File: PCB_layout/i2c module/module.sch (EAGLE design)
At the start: 5 parts, among them IC1 ATTINY85-20SU, J1 M20-9980346

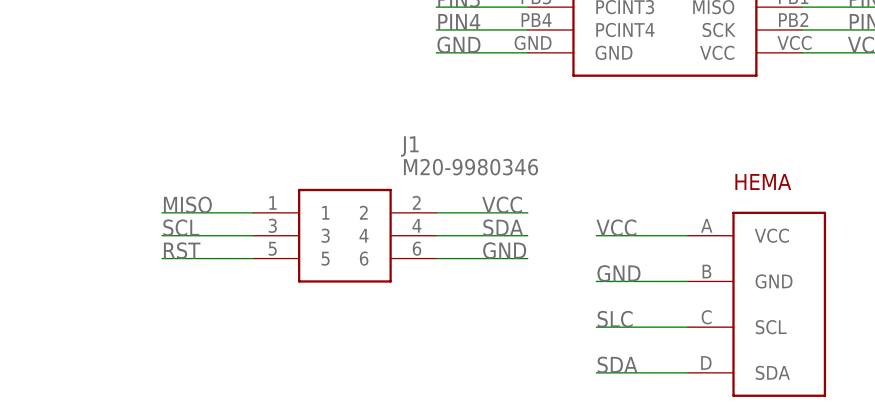
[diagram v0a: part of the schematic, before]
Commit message: i2c, lbr updates
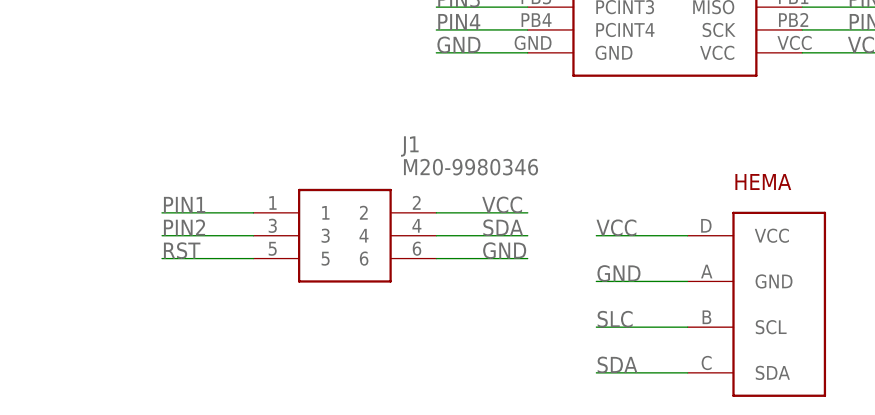
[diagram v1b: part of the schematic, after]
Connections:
- removed net MISO: J1.1
- removed net SCL: J1.3
- net PIN1: now also J1.1
- net PIN2: now also J1.3
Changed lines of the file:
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@@
-</segment>
-</net>
-<net name="MISO" class="0">
-<segment>
-<pinref part="J1" gate="G$1" pin="1"/>
-<wire x1="5.08" y1="58.42" x2="-5.08" y2="58.42" width="0.1524" layer="91"/>
-<label x="-5.08" y="58.42" size="1.778" layer="95"/>
-</segment>
-</net>
-<net name="SCL" class="0">
-<segment>
-<pinref part="J1" gate="G$1" pin="3"/>
-<wire x1="5.08" y1="55.88" x2="-5.08" y2="55.88" width="0.1524" layer="91"/>
-<label x="-5.08" y="55.88" size="1.778" layer="95"/>
 </segment>
 </net>
@@
 <label x="71.12" y="81.28" size="1.778" layer="95"/>
 </segment>
+<segment>
+<pinref part="J1" gate="G$1" pin="1"/>
+<wire x1="5.08" y1="58.42" x2="-5.08" y2="58.42" width="0.1524" layer="91"/>
+<label x="-5.08" y="58.42" size="1.778" layer="95"/>
+</segment>
 </net>
 <net name="PIN2" class="0">
@@
 <wire x1="66.04" y1="78.74" x2="76.2" y2="78.74" width="0.1524" layer="91"/>
 <label x="71.12" y="78.74" size="1.778" layer="95"/>
+</segment>
+<segment>
+<pinref part="J1" gate="G$1" pin="3"/>
+<wire x1="5.08" y1="55.88" x2="-5.08" y2="55.88" width="0.1524" layer="91"/>
+<label x="-5.08" y="55.88" size="1.778" layer="95"/>
 </segment>
 </net>
@@
 </drawing>
 <compatibility>
+<note version="6.3" minversion="6.2.2" severity="warning">
+Since Version 6.2.2 text objects can contain more than one line,
+which will not be processed correctly with this version.
+</note>
 <note version="8.2" severity="warning">
 Since Version 8.2, EAGLE supports online libraries. The ids

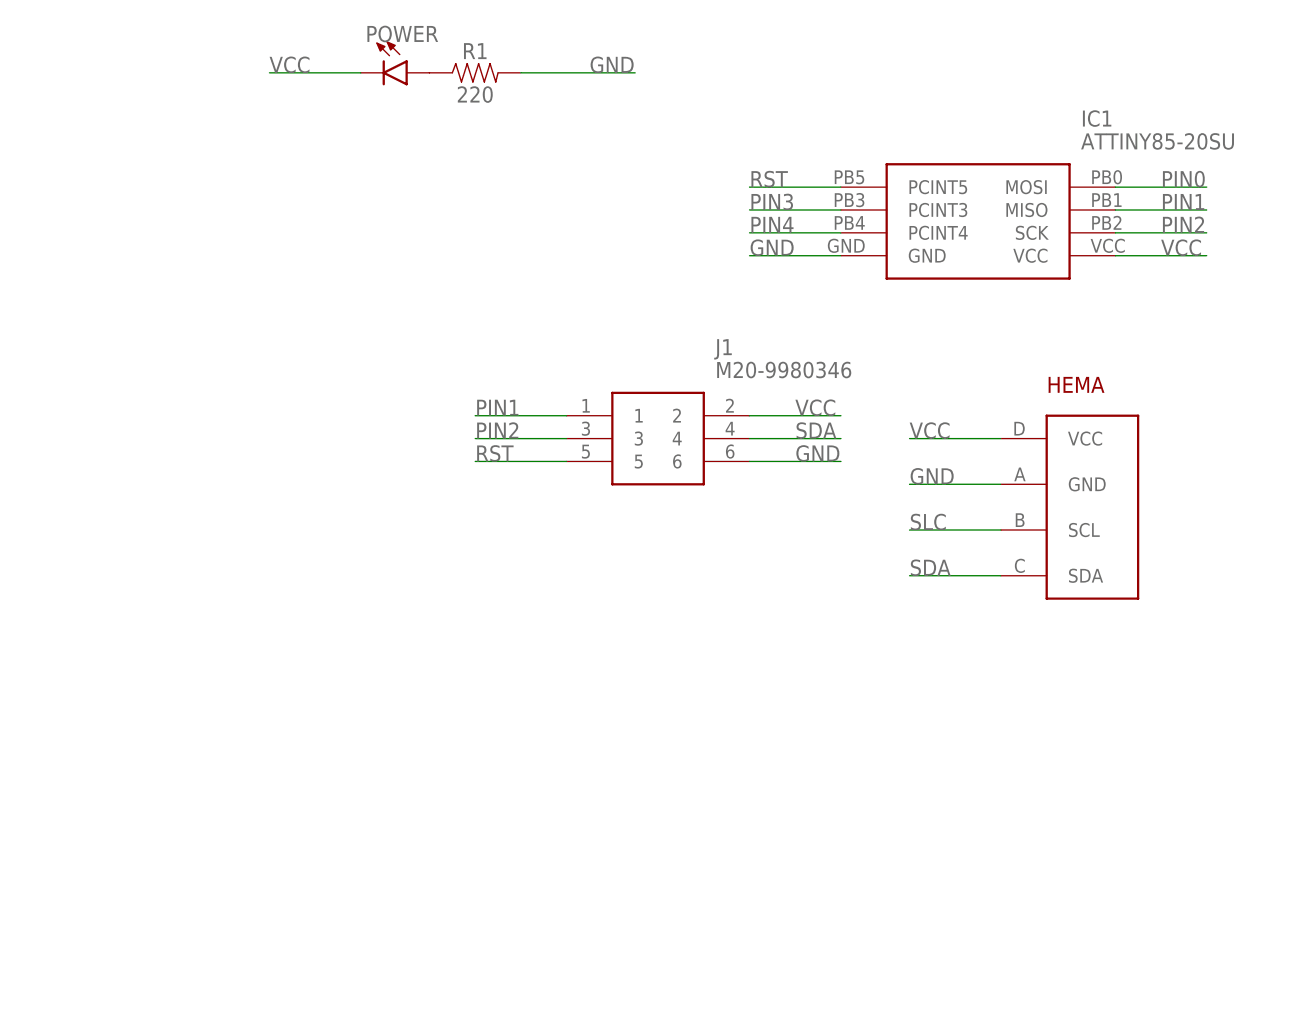
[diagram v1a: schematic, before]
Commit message: PCB design/lib updates
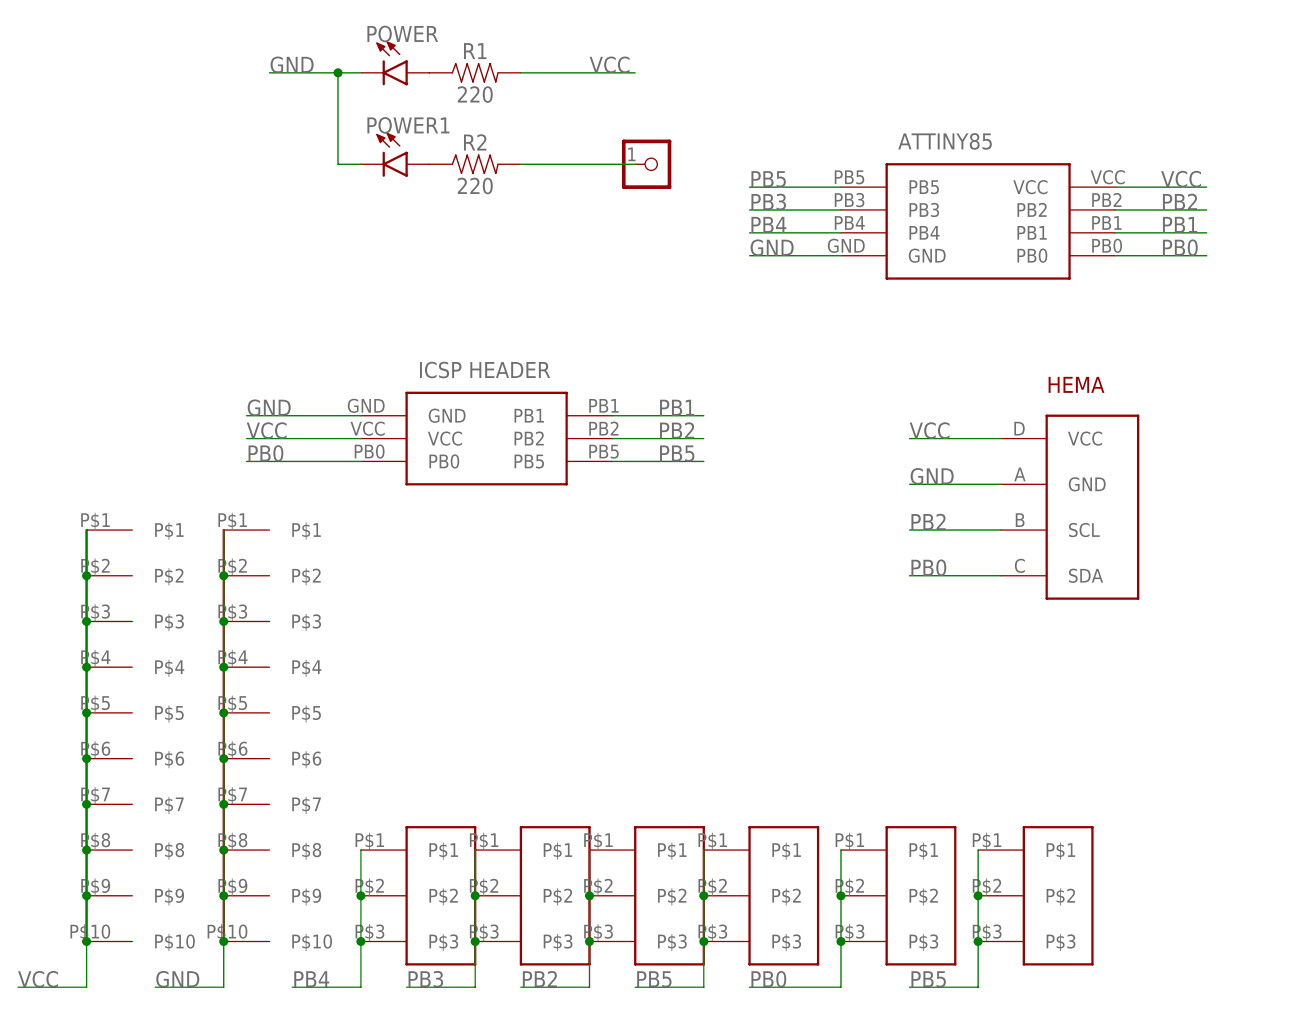
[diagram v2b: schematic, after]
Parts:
- added 0, 1, 2, 3, 4, 5: 3X-PADS-CONNECTED, BadgeParts:3X-PADS-CONNECTED
- added GND, VCC: 10X-PADS, BadgeParts:10X-PADS
- added P1: PROTO_VIAS_01X01-1.2, dp_devices:PROTO_VIAS_01X01-1.2
- added POWER1: (no value), SparkFun-LED:LED3MM
- added R2: 220, SparkFun-Resistors:RESISTORAXIAL-0.3
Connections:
- removed net PIN0: IC1.MOSI
- removed net PIN1: IC1.MISO, J1.1
- removed net PIN2: IC1.SCK, J1.3
- removed net PIN3: IC1.PCINT3
- removed net PIN4: IC1.PCINT4
- removed net RST: IC1.PCINT5, J1.5
- removed net SDA: J1.4, U$1.SDA
- removed net SLC: U$1.SCL
- new net N$1: POWER1.A, R2.1
- new net N$2: P1.1, R2.2
- new net PB0: 0.P$1, 0.P$2, 0.P$3, IC1.PB0, J1.PB0, U$1.SDA
- new net PB1: IC1.PB1, J1.PB1
- new net PB2: 2.P$1, 2.P$2, 2.P$3, IC1.PB2, J1.PB2, U$1.SCL
- new net PB3: 3.P$1, 3.P$2, 3.P$3, IC1.PB3
- new net PB4: 4.P$1, 4.P$2, 4.P$3, IC1.PB4
- new net PB5: 1.P$1, 1.P$2, 1.P$3, 5.P$1, 5.P$2, 5.P$3, IC1.PB5, J1.PB5
- net GND: now also GND.P$1, GND.P$10, GND.P$2, GND.P$3, GND.P$4, GND.P$5, GND.P$6, GND.P$7, GND.P$8, GND.P$9, J1.GND, POWER.C, POWER1.C; no longer J1.6, R1.2
- net VCC: now also J1.VCC, R1.2, VCC.P$1, VCC.P$10, VCC.P$2, VCC.P$3, VCC.P$4, VCC.P$5, VCC.P$6, VCC.P$7, VCC.P$8, VCC.P$9; no longer J1.2, POWER.C

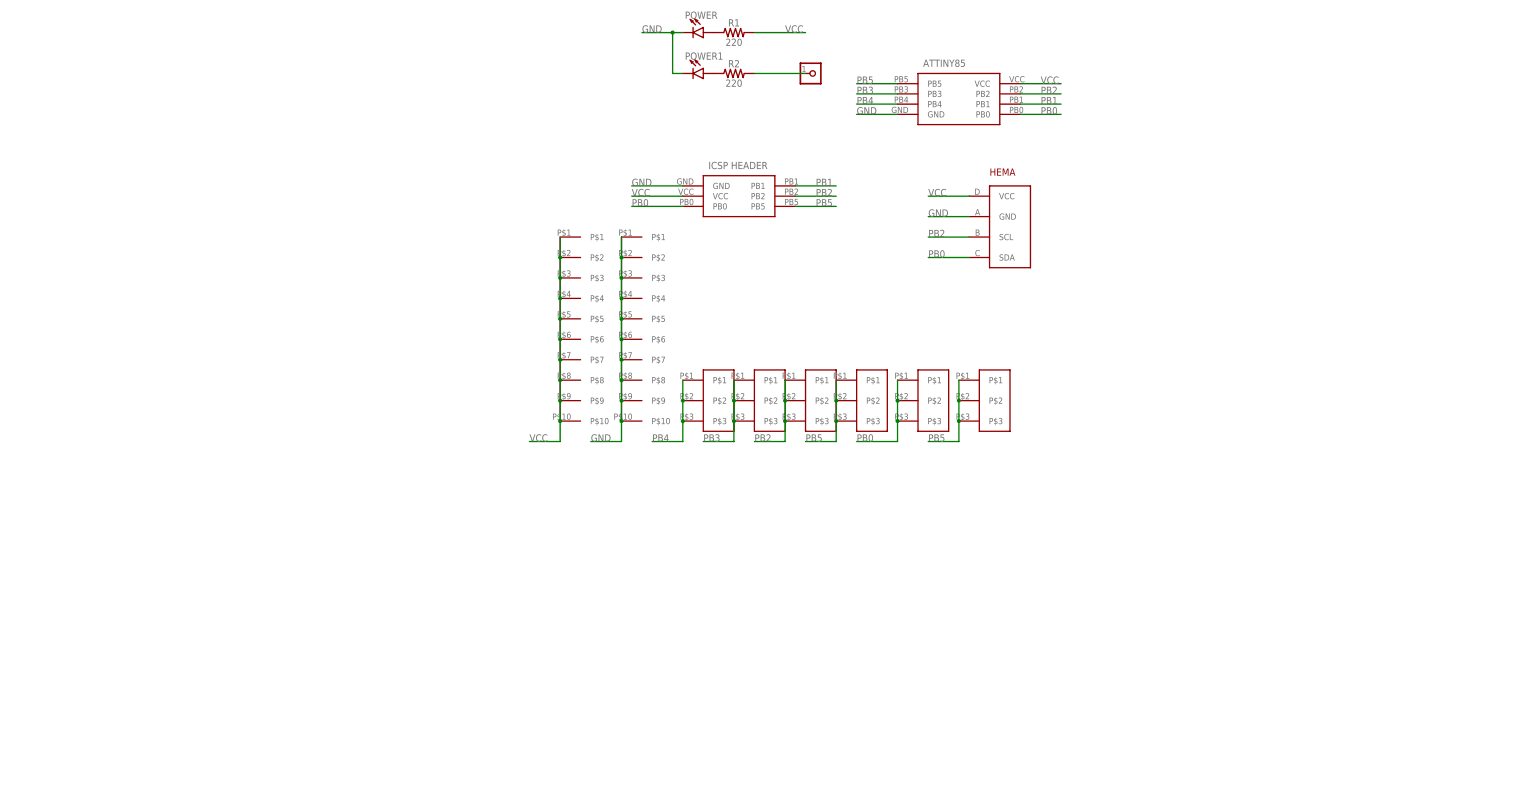
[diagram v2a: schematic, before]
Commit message: first i2c dongle iteration panelized
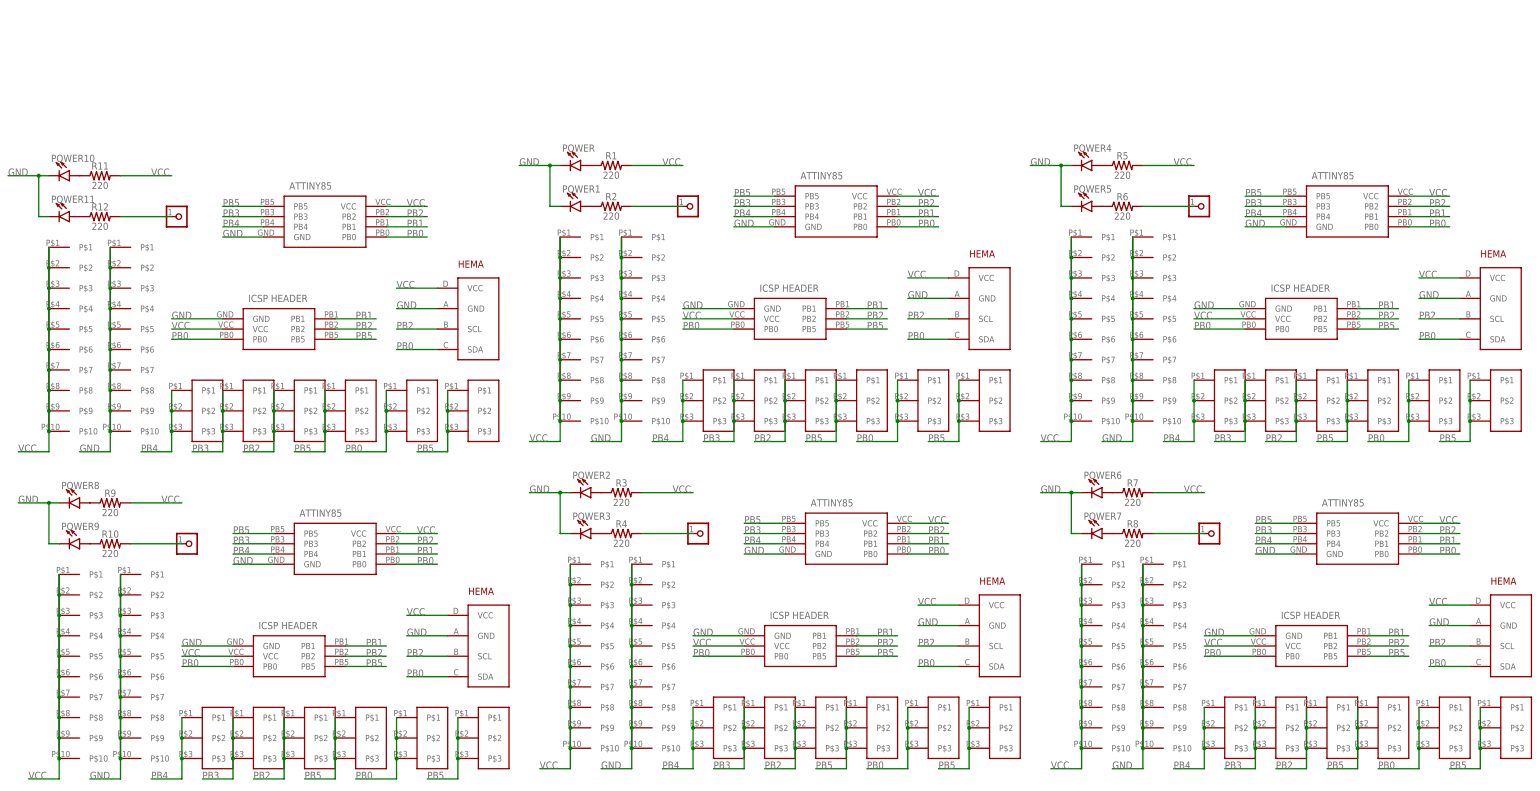
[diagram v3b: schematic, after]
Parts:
- added 10, 11, 12, 13, 14, 15, 16, 17, 18, 19, 20, 21, 22, 23, 24, 25, 26, 27, 28, 29, 30, 31, 32, 33, 34, 35, 6, 7, 8, 9: 3X-PADS-CONNECTED, BadgeParts:3X-PADS-CONNECTED
- added GND1, GND2, GND3, GND4, GND5, VCC1, VCC2, VCC3, VCC4, VCC5: 10X-PADS, BadgeParts:10X-PADS
- added IC2, IC3, IC4, IC5, IC6: ATTINY85-20SU, BadgeParts:ATTINY85-20SU
- added J2, J3, J4, J5, J6: M20-9980346, BadgeParts:M20-9980346
- added P2, P3, P4, P5, P6: PROTO_VIAS_01X01-1.2, dp_devices:PROTO_VIAS_01X01-1.2
- added POWER10, POWER11, POWER2, POWER3, POWER4, POWER5, POWER6, POWER7, POWER8, POWER9: (no value), SparkFun-LED:LED3MM
- added R10, R11, R12, R3, R4, R5, R6, R7, R8, R9: 220, SparkFun-Resistors:RESISTORAXIAL-0.3
- added U$2, U$3, U$4, U$5, U$6: HEMA-I2C, BadgeParts:HEMA-I2C
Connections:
- new net N$10: POWER7.A, R8.1
- new net N$12: P4.1, R8.2
- new net N$13: POWER8.A, R9.1
- new net N$14: POWER9.A, R10.1
- new net N$15: P5.1, R10.2
- new net N$16: POWER10.A, R11.1
- new net N$17: POWER11.A, R12.1
- new net N$18: P6.1, R12.2
- new net N$3: POWER2.A, R3.1
- new net N$4: POWER3.A, R4.1
- new net N$5: P2.1, R4.2
- new net N$6: POWER4.A, R5.1
- new net N$7: POWER5.A, R6.1
- new net N$8: P3.1, R6.2
- new net N$9: POWER6.A, R7.1
- net GND: now also GND1.P$1, GND1.P$10, GND1.P$2, GND1.P$3, GND1.P$4, GND1.P$5, GND1.P$6, GND1.P$7, GND1.P$8, GND1.P$9, GND2.P$1, GND2.P$10, GND2.P$2, GND2.P$3, GND2.P$4, GND2.P$5, GND2.P$6, GND2.P$7, GND2.P$8, GND2.P$9, GND3.P$1, GND3.P$10, GND3.P$2, GND3.P$3, GND3.P$4, GND3.P$5, GND3.P$6, GND3.P$7, GND3.P$8, GND3.P$9, GND4.P$1, GND4.P$10, GND4.P$2, GND4.P$3, GND4.P$4, GND4.P$5, GND4.P$6, GND4.P$7, GND4.P$8, GND4.P$9, GND5.P$1, GND5.P$10, GND5.P$2, GND5.P$3, GND5.P$4, GND5.P$5, GND5.P$6, GND5.P$7, GND5.P$8, GND5.P$9, IC2.GND, IC3.GND, IC4.GND, IC5.GND, IC6.GND, J2.GND, J3.GND, J4.GND, J5.GND, J6.GND, POWER10.C, POWER11.C, POWER2.C, POWER3.C, POWER4.C, POWER5.C, POWER6.C, POWER7.C, POWER8.C, POWER9.C, U$2.GND, U$3.GND, U$4.GND, U$5.GND, U$6.GND
- net PB0: now also 10.P$1, 10.P$2, 10.P$3, 16.P$1, 16.P$2, 16.P$3, 22.P$1, 22.P$2, 22.P$3, 28.P$1, 28.P$2, 28.P$3, 34.P$1, 34.P$2, 34.P$3, IC2.PB0, IC3.PB0, IC4.PB0, IC5.PB0, IC6.PB0, J2.PB0, J3.PB0, J4.PB0, J5.PB0, J6.PB0, U$2.SDA, U$3.SDA, U$4.SDA, U$5.SDA, U$6.SDA
- net PB1: now also IC2.PB1, IC3.PB1, IC4.PB1, IC5.PB1, IC6.PB1, J2.PB1, J3.PB1, J4.PB1, J5.PB1, J6.PB1
- net PB2: now also 14.P$1, 14.P$2, 14.P$3, 20.P$1, 20.P$2, 20.P$3, 26.P$1, 26.P$2, 26.P$3, 32.P$1, 32.P$2, 32.P$3, 8.P$1, 8.P$2, 8.P$3, IC2.PB2, IC3.PB2, IC4.PB2, IC5.PB2, IC6.PB2, J2.PB2, J3.PB2, J4.PB2, J5.PB2, J6.PB2, U$2.SCL, U$3.SCL, U$4.SCL, U$5.SCL, U$6.SCL
- net PB3: now also 13.P$1, 13.P$2, 13.P$3, 19.P$1, 19.P$2, 19.P$3, 25.P$1, 25.P$2, 25.P$3, 31.P$1, 31.P$2, 31.P$3, 7.P$1, 7.P$2, 7.P$3, IC2.PB3, IC3.PB3, IC4.PB3, IC5.PB3, IC6.PB3
- net PB4: now also 12.P$1, 12.P$2, 12.P$3, 18.P$1, 18.P$2, 18.P$3, 24.P$1, 24.P$2, 24.P$3, 30.P$1, 30.P$2, 30.P$3, 6.P$1, 6.P$2, 6.P$3, IC2.PB4, IC3.PB4, IC4.PB4, IC5.PB4, IC6.PB4
- net PB5: now also 11.P$1, 11.P$2, 11.P$3, 15.P$1, 15.P$2, 15.P$3, 17.P$1, 17.P$2, 17.P$3, 21.P$1, 21.P$2, 21.P$3, 23.P$1, 23.P$2, 23.P$3, 27.P$1, 27.P$2, 27.P$3, 29.P$1, 29.P$2, 29.P$3, 33.P$1, 33.P$2, 33.P$3, 35.P$1, 35.P$2, 35.P$3, 9.P$1, 9.P$2, 9.P$3, IC2.PB5, IC3.PB5, IC4.PB5, IC5.PB5, IC6.PB5, J2.PB5, J3.PB5, J4.PB5, J5.PB5, J6.PB5
- net VCC: now also IC2.VCC, IC3.VCC, IC4.VCC, IC5.VCC, IC6.VCC, J2.VCC, J3.VCC, J4.VCC, J5.VCC, J6.VCC, R11.2, R3.2, R5.2, R7.2, R9.2, U$2.VCC, U$3.VCC, U$4.VCC, U$5.VCC, U$6.VCC, VCC1.P$1, VCC1.P$10, VCC1.P$2, VCC1.P$3, VCC1.P$4, VCC1.P$5, VCC1.P$6, VCC1.P$7, VCC1.P$8, VCC1.P$9, VCC2.P$1, VCC2.P$10, VCC2.P$2, VCC2.P$3, VCC2.P$4, VCC2.P$5, VCC2.P$6, VCC2.P$7, VCC2.P$8, VCC2.P$9, VCC3.P$1, VCC3.P$10, VCC3.P$2, VCC3.P$3, VCC3.P$4, VCC3.P$5, VCC3.P$6, VCC3.P$7, VCC3.P$8, VCC3.P$9, VCC4.P$1, VCC4.P$10, VCC4.P$2, VCC4.P$3, VCC4.P$4, VCC4.P$5, VCC4.P$6, VCC4.P$7, VCC4.P$8, VCC4.P$9, VCC5.P$1, VCC5.P$10, VCC5.P$2, VCC5.P$3, VCC5.P$4, VCC5.P$5, VCC5.P$6, VCC5.P$7, VCC5.P$8, VCC5.P$9
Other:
- moved on the sheet: POWER, POWER1, R1, R2
